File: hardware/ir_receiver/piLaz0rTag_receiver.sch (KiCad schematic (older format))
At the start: 4 parts, among them U1 TSOP4838

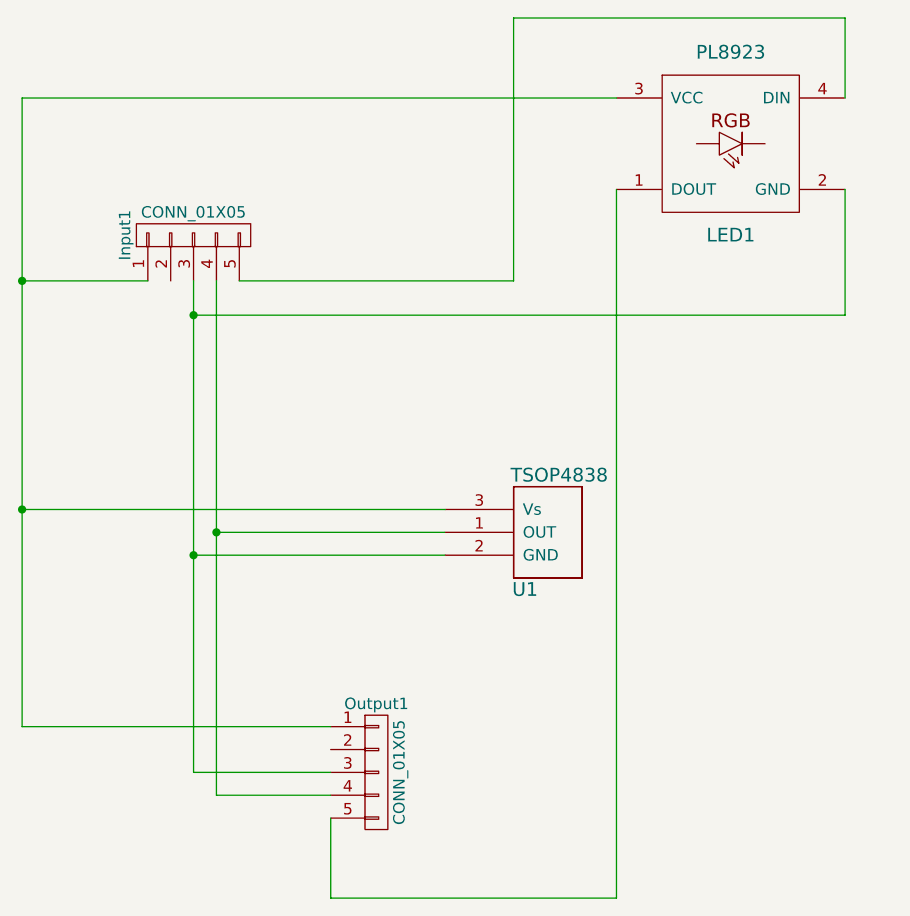
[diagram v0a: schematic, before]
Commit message: #9 Ir Receiver
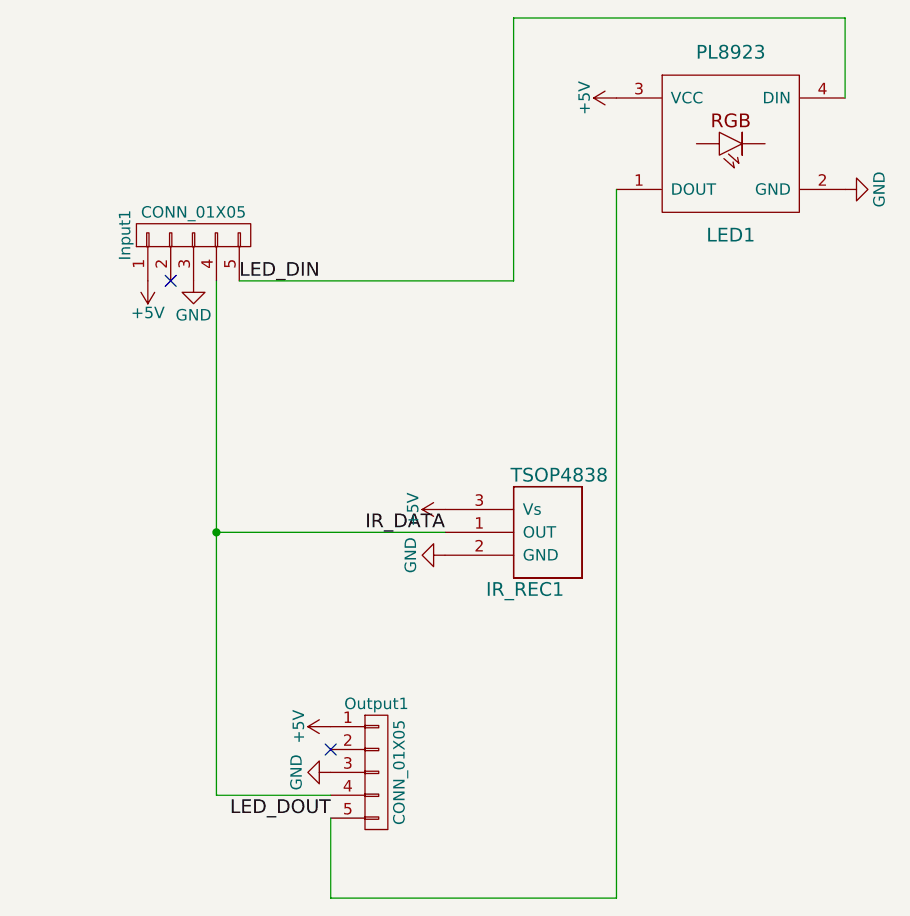
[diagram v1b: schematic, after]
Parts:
- renumbered U1 to IR_REC1
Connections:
- net IR_DATA: now reaches IR_REC1.1 (OUT), Input1.4 (P4), Output1.4 (P4)
- net GND: now reaches IR_REC1.2 (GND), Input1.3 (P3), LED1.2 (GND), Output1.3 (P3)
- net +5V: now reaches IR_REC1.3 (Vs), Input1.1 (P1), LED1.3 (VCC), Output1.1 (P1)
- net LED_DIN: now reaches Input1.5 (P5), LED1.4 (DIN)
- net LED_DOUT: now reaches LED1.1 (DOUT), Output1.5 (P5)
- no-connect marks 0 -> 2
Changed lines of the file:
@@
 $EndDescr
 $Comp
-L TSOP4838 U1
+L TSOP4838 IR_REC1
 U 1 1 58F39155
 P 3400 2850
-F 0 "U1" H 3300 2600 60  0000 C CNN
+F 0 "IR_REC1" H 3300 2600 60  0000 C CNN
 F 1 "TSOP4838" H 3450 3100 60  0000 C CNN
 F 2 "Opto-Devices:IRReceiver_Vishay_MOLD-3pin" H 3400 2850 60  0001 C CNN
@@
 	1    0    0    -1
 $EndComp
-Wire Wire Line
-	1650 1750 1100 1750
-Wire Wire Line
-	1100 950  1100 3700
-Wire Wire Line
-	1100 950  3700 950
-Wire Wire Line
-	1850 1750 1850 3900
-Wire Wire Line
-	1850 1900 4700 1900
-Wire Wire Line
-	4700 1900 4700 1350
-Wire Wire Line
-	1850 2950 2950 2950
-Connection ~ 1850 1900
-Wire Wire Line
-	1100 2750 2950 2750
-Connection ~ 1100 1750
-Wire Wire Line
-	1100 3700 2450 3700
-Connection ~ 1100 2750
-Wire Wire Line
-	1850 3900 2450 3900
-Connection ~ 1850 2950
 Wire Wire Line
 	1950 1750 1950 4000
@@
 	1    0    0    -1
 $EndComp
+NoConn ~ 1750 1750
+NoConn ~ 2450 3800
+$Comp
+L GND #PWR01
+U 1 1 590CA84F
+P 2450 3900
+F 0 "#PWR01" H 2450 3650 50  0001 C CNN
+F 1 "GND" H 2450 3750 50  0000 C CNN
+F 2 "" H 2450 3900 50  0001 C CNN
+F 3 "" H 2450 3900 50  0001 C CNN
+	1    2450 3900
+	0    1    1    0
+$EndComp
+$Comp
+L GND #PWR02
+U 1 1 590CA8D5
+P 2950 2950
+F 0 "#PWR02" H 2950 2700 50  0001 C CNN
+F 1 "GND" H 2950 2800 50  0000 C CNN
+F 2 "" H 2950 2950 50  0001 C CNN
+F 3 "" H 2950 2950 50  0001 C CNN
+	1    2950 2950
+	0    1    1    0
+$EndComp
+$Comp
+L GND #PWR03
+U 1 1 590CA905
+P 4700 1350
+F 0 "#PWR03" H 4700 1100 50  0001 C CNN
+F 1 "GND" H 4700 1200 50  0000 C CNN
+F 2 "" H 4700 1350 50  0001 C CNN
+F 3 "" H 4700 1350 50  0001 C CNN
+	1    4700 1350
+	0    -1   -1   0
+$EndComp
+$Comp
+L GND #PWR04
+U 1 1 590CA921
+P 1850 1750
+F 0 "#PWR04" H 1850 1500 50  0001 C CNN
+F 1 "GND" H 1850 1600 50  0000 C CNN
+F 2 "" H 1850 1750 50  0001 C CNN
+F 3 "" H 1850 1750 50  0001 C CNN
+	1    1850 1750
+	1    0    0    -1
+$EndComp
+$Comp
+L +5V #PWR05
+U 1 1 590CA9D7
+P 1650 1750
+F 0 "#PWR05" H 1650 1600 50  0001 C CNN
+F 1 "+5V" H 1650 1890 50  0000 C CNN
+F 2 "" H 1650 1750 50  0001 C CNN
+F 3 "" H 1650 1750 50  0001 C CNN
+	1    1650 1750
+	-1   0    0    1
+$EndComp
+$Comp
+L +5V #PWR06
+U 1 1 590CAA28
+P 2450 3700
+F 0 "#PWR06" H 2450 3550 50  0001 C CNN
+F 1 "+5V" H 2450 3840 50  0000 C CNN
+F 2 "" H 2450 3700 50  0001 C CNN
+F 3 "" H 2450 3700 50  0001 C CNN
+	1    2450 3700
+	0    -1   -1   0
+$EndComp
+$Comp
+L +5V #PWR07
+U 1 1 590CAA44
+P 3700 950
+F 0 "#PWR07" H 3700 800 50  0001 C CNN
+F 1 "+5V" H 3700 1090 50  0000 C CNN
+F 2 "" H 3700 950 50  0001 C CNN
+F 3 "" H 3700 950 50  0001 C CNN
+	1    3700 950
+	0    -1   -1   0
+$EndComp
+$Comp
+L +5V #PWR08
+U 1 1 590CAAB3
+P 2950 2750
+F 0 "#PWR08" H 2950 2600 50  0001 C CNN
+F 1 "+5V" H 2950 2890 50  0000 C CNN
+F 2 "" H 2950 2750 50  0001 C CNN
+F 3 "" H 2950 2750 50  0001 C CNN
+	1    2950 2750
+	0    -1   -1   0
+$EndComp
+Text Label 2050 1750 0    60   ~ 0
+LED_DIN
+Text Label 2450 4100 2    60   ~ 0
+LED_DOUT
+Text Label 2950 2850 2    60   ~ 0
+IR_DATA
 $EndSCHEMATC

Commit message: Some minor changes on the receiver mainboard
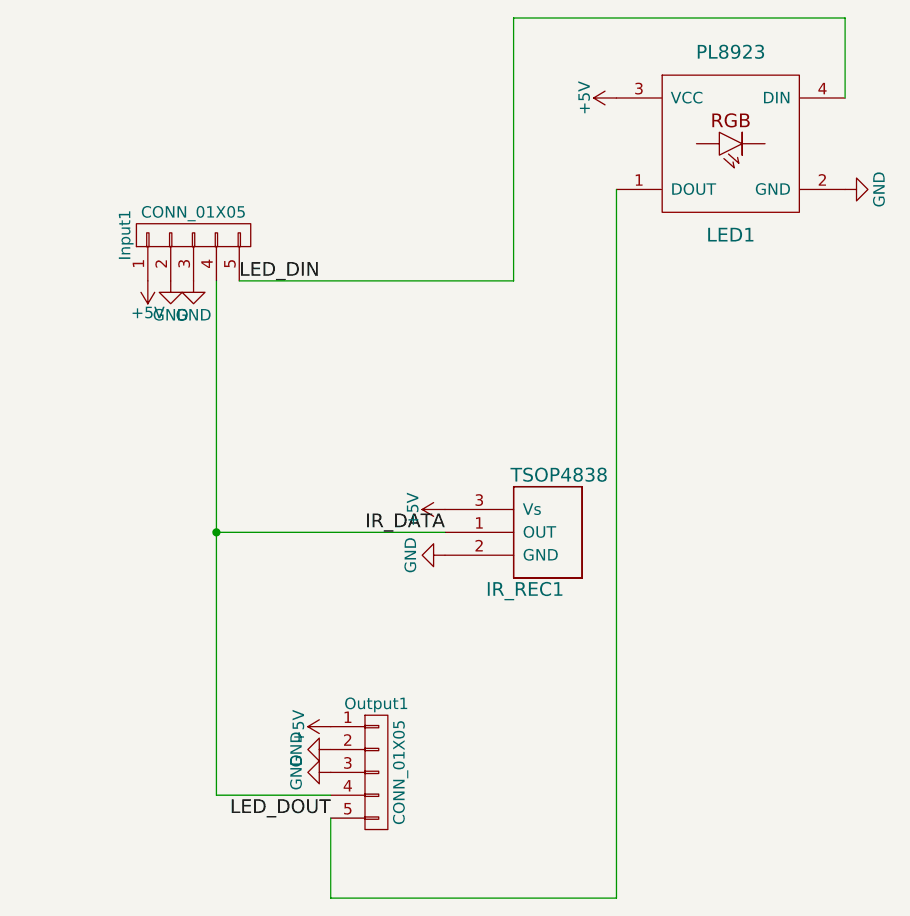
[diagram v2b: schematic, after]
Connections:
- net GND: now also Input1.2 (P2), Output1.2 (P2)
- no-connect marks 2 -> 0
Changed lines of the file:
@@
 	1    0    0    -1
 $EndComp
-NoConn ~ 1750 1750
-NoConn ~ 2450 3800
 $Comp
 L GND #PWR01
@@
 Text Label 2950 2850 2    60   ~ 0
 IR_DATA
+$Comp
+L GND #PWR?
+U 1 1 590DBFD1
+P 2450 3800
+F 0 "#PWR?" H 2450 3550 50  0001 C CNN
+F 1 "GND" H 2450 3650 50  0000 C CNN
+F 2 "" H 2450 3800 50  0001 C CNN
+F 3 "" H 2450 3800 50  0001 C CNN
+	1    2450 3800
+	0    1    1    0
+$EndComp
+$Comp
+L GND #PWR?
+U 1 1 590DBFED
+P 1750 1750
+F 0 "#PWR?" H 1750 1500 50  0001 C CNN
+F 1 "GND" H 1750 1600 50  0000 C CNN
+F 2 "" H 1750 1750 50  0001 C CNN
+F 3 "" H 1750 1750 50  0001 C CNN
+	1    1750 1750
+	1    0    0    -1
+$EndComp
 $EndSCHEMATC
